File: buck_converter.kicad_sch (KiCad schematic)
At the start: 19 parts, among them Q5 CSD17579Q3A, Q6 CSD17579Q3A, U5 TPS40305DRCR

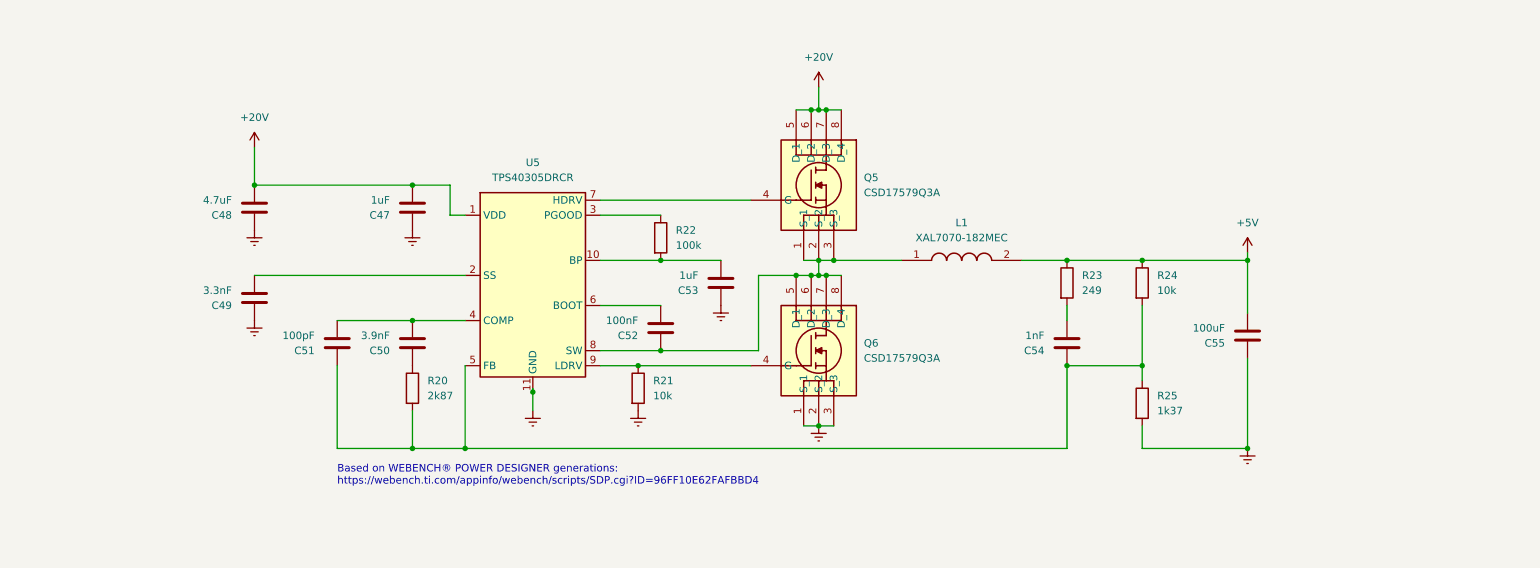
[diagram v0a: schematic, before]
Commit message: some new ideas for power
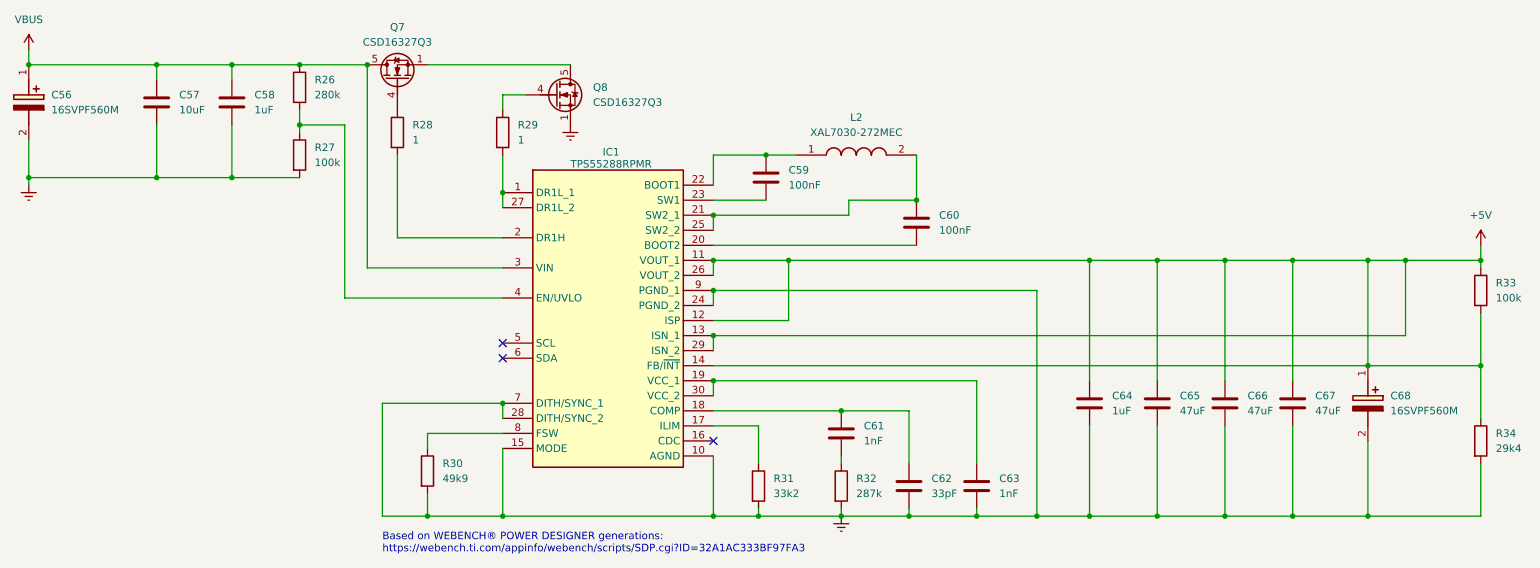
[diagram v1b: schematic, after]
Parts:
- removed C47, C53: 1uF, Capacitor_SMD:C_0603_1608Metric_Pad1.08x0.95mm_HandSolder, symbol Device:C
- removed C48: 4.7uF, Capacitor_SMD:C_0603_1608Metric_Pad1.08x0.95mm_HandSolder, symbol Device:C
- removed C49: 3.3nF, Capacitor_SMD:C_0603_1608Metric_Pad1.08x0.95mm_HandSolder, symbol Device:C
- removed C50: 3.9nF, Capacitor_SMD:C_0603_1608Metric_Pad1.08x0.95mm_HandSolder, symbol Device:C
- removed C51: 100pF, Capacitor_SMD:C_0603_1608Metric_Pad1.08x0.95mm_HandSolder, symbol Device:C
- removed C52: 100nF, Capacitor_SMD:C_0603_1608Metric_Pad1.08x0.95mm_HandSolder, symbol Device:C
- removed C54: 1nF, Capacitor_SMD:C_0603_1608Metric_Pad1.08x0.95mm_HandSolder, symbol Device:C
- removed C55: 100uF, Capacitor_SMD:C_0603_1608Metric_Pad1.08x0.95mm_HandSolder, symbol Device:C
- removed L1: XAL7070-182MEC, INDC7275X700N, symbol XAL7070-182MEC:XAL7070-182MEC
- removed Q5, Q6: CSD17579Q3A, Q3A, symbol CSD17579Q3A:CSD17579Q3A
- removed R20: 2k87, Resistor_SMD:R_0603_1608Metric_Pad0.98x0.95mm_HandSolder, symbol Device:R
- removed R21, R24: 10k, Resistor_SMD:R_0603_1608Metric_Pad0.98x0.95mm_HandSolder, symbol Device:R
- removed R22: 100k, Resistor_SMD:R_0603_1608Metric_Pad0.98x0.95mm_HandSolder, symbol Device:R
- removed R23: 249, Resistor_SMD:R_0603_1608Metric_Pad0.98x0.95mm_HandSolder, symbol Device:R
- removed R25: 1k37, Resistor_SMD:R_0603_1608Metric_Pad0.98x0.95mm_HandSolder, symbol Device:R
- removed U5: TPS40305DRCR, Package_SON:Texas_DRC0010J_ThermalVias, symbol New_Library:TPS40305DRCR
- added C56: 16SVPF560M, 16SVPT560M, symbol 16SVPF560M:16SVPF560M
- added C57: 10uF, Capacitor_SMD:C_1210_3225Metric_Pad1.33x2.70mm_HandSolder, symbol Device:C
- added C58: 1uF, Capacitor_SMD:C_0402_1005Metric_Pad0.74x0.62mm_HandSolder, symbol Device:C
- added C59, C60: 100nF, Capacitor_SMD:C_0603_1608Metric_Pad1.08x0.95mm_HandSolder, symbol Device:C
- added C61: 1nF, Capacitor_SMD:C_0402_1005Metric_Pad0.74x0.62mm_HandSolder, symbol Device:C
- added C62: 33pF, Capacitor_SMD:C_0402_1005Metric_Pad0.74x0.62mm_HandSolder, symbol Device:C
- added C63: 1nF, Capacitor_SMD:C_0603_1608Metric_Pad1.08x0.95mm_HandSolder, symbol Device:C
- added C64: 1uF, Capacitor_SMD:C_0603_1608Metric_Pad1.08x0.95mm_HandSolder, symbol Device:C
- added C65, C66, C67: 47uF, Capacitor_SMD:C_1210_3225Metric_Pad1.33x2.70mm_HandSolder, symbol Device:C
- added C68: 16SVPF560M, 16SVPF560M:16SVPT560M, symbol 16SVPF560M:16SVPF560M
- added IC1: TPS55288RPMR, TPS55288RPMR, symbol TPS55288RPMR:TPS55288RPMR
- added L2: XAL7030-272MEC, XAL7030-272MEC:XAL7030272MEC, symbol XAL7030-272MEC:XAL7030-272MEC
- added Q7, Q8: CSD16327Q3, Package_SON:VSON-8_3.3x3.3mm_P0.65mm_NexFET, symbol Transistor_FET:CSD16327Q3
- added R26: 280k, Resistor_SMD:R_0603_1608Metric_Pad0.98x0.95mm_HandSolder, symbol Device:R
- added R27, R33: 100k, Resistor_SMD:R_0603_1608Metric_Pad0.98x0.95mm_HandSolder, symbol Device:R
- added R28, R29: 1, Resistor_SMD:R_0603_1608Metric_Pad0.98x0.95mm_HandSolder, symbol Device:R
- added R30: 49k9, Resistor_SMD:R_0603_1608Metric_Pad0.98x0.95mm_HandSolder, symbol Device:R
- added R31: 33k2, Resistor_SMD:R_0603_1608Metric_Pad0.98x0.95mm_HandSolder, symbol Device:R
- added R32: 287k, Resistor_SMD:R_0603_1608Metric_Pad0.98x0.95mm_HandSolder, symbol Device:R
- added R34: 29k4, Resistor_SMD:R_0603_1608Metric_Pad0.98x0.95mm_HandSolder, symbol Device:R
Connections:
- net +5V: now also C64.1, C65.1, C66.1, C67.1, C68.1 (+), IC1.11 (VOUT_1), IC1.12 (ISP), IC1.13 (ISN_1), IC1.14 (FB/~{INT}), IC1.26 (VOUT_2), IC1.29 (ISN_2), R33.1, R33.2, R34.1
- net GND: now also C56.2 (-), C57.2, C58.2, C62.2, C63.2, C64.2, C65.2, C66.2, C67.2, C68.2 (-), IC1.10 (AGND), IC1.15 (MODE), IC1.24 (PGND_2), IC1.28 (DITH/SYNC_2), IC1.7 (DITH/SYNC_1), IC1.9 (PGND_1), Q8.1 (S), Q8.2 (S), Q8.3 (S), R27.2, R30.2, R31.2, R32.2, R34.2
- new net: IC1.17 (ILIM), R31.1
- new net: C61.2, R32.1
- new net: C61.1, C62.1, IC1.18 (COMP)
- new net: Q7.4 (G), R28.1
- new net: IC1.2 (DR1H), R28.2
- new net: C59.1, IC1.22 (BOOT1), L2.1
- new net: C59.2, IC1.23 (SW1)
- new net: IC1.8 (FSW), R30.1
- new net: IC1.4 (EN/UVLO), R26.2, R27.1
- new net: IC1.1 (DR1L_1), IC1.27 (DR1L_2), R29.2
- new net: C63.1, IC1.19 (VCC_1), IC1.30 (VCC_2)
- new net: C60.2, IC1.20 (BOOT2)
- new net: C60.1, IC1.21 (SW2_1), IC1.25 (SW2_2), L2.2
- new net: Q8.4 (G), R29.1
- new net: Q7.1 (S), Q7.2 (S), Q7.3 (S), Q8.5 (D)
- new net VBUS: C56.1 (+), C57.1, C58.1, IC1.3 (VIN), Q7.5 (D), R26.1
- no-connect marks 0 -> 3
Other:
- note added: "Based on WEBENCH® POWER DESIGNER generations: https://webench.ti.com/appinfo/webench/scripts/SDP.cgi?ID=32A1AC333BF97FA3"
- note removed: "Based on WEBENCH® POWER DESIGNER generations: https://webench.ti.com/appinfo/webench/scripts/SDP.cgi?ID=96FF10E62FAFBBD4"
